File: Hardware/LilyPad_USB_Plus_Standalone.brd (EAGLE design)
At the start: 50.7 x 50.7 mm, 101 parts, among them J1 SEWTAP_LONG-2SIDE, J10 SEWTAP_LONG-2SIDE, J11 SEWTAP_LONG-2SIDE, J12 SEWTAP_LONG-2SIDE, J13 SEWTAP_LONG-2SIDE, J14 SEWTAP_LONG-2SIDE, J15 AMP FCI 10103594-0001LF, J2 SEWTAP_LONG-2SIDE, J3 SEWTAP_LONG-2SIDE, J4 SEWTAP_LONG-2SIDE, J5 SEWTAP_LONG-2SIDE, J6 SEWTAP_LONG-2SIDE, J7 SEWTAP_LONG-2SIDE, J8 SEWTAP_LONG-2SIDE, J9 SEWTAP_LONG-2SIDE, U1 MCP73831, U2 3.3V, U5 32U4, Y1 8MHz

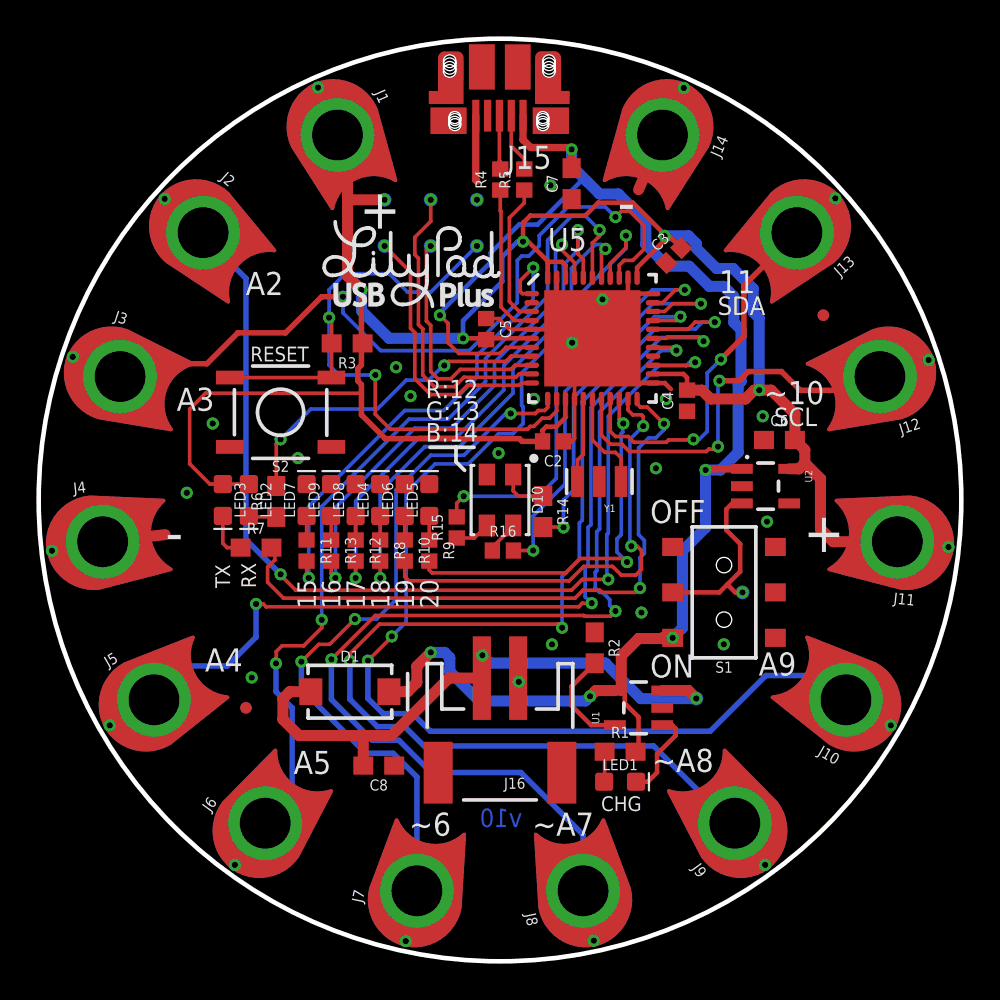
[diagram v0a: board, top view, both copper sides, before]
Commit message: Changes after double check
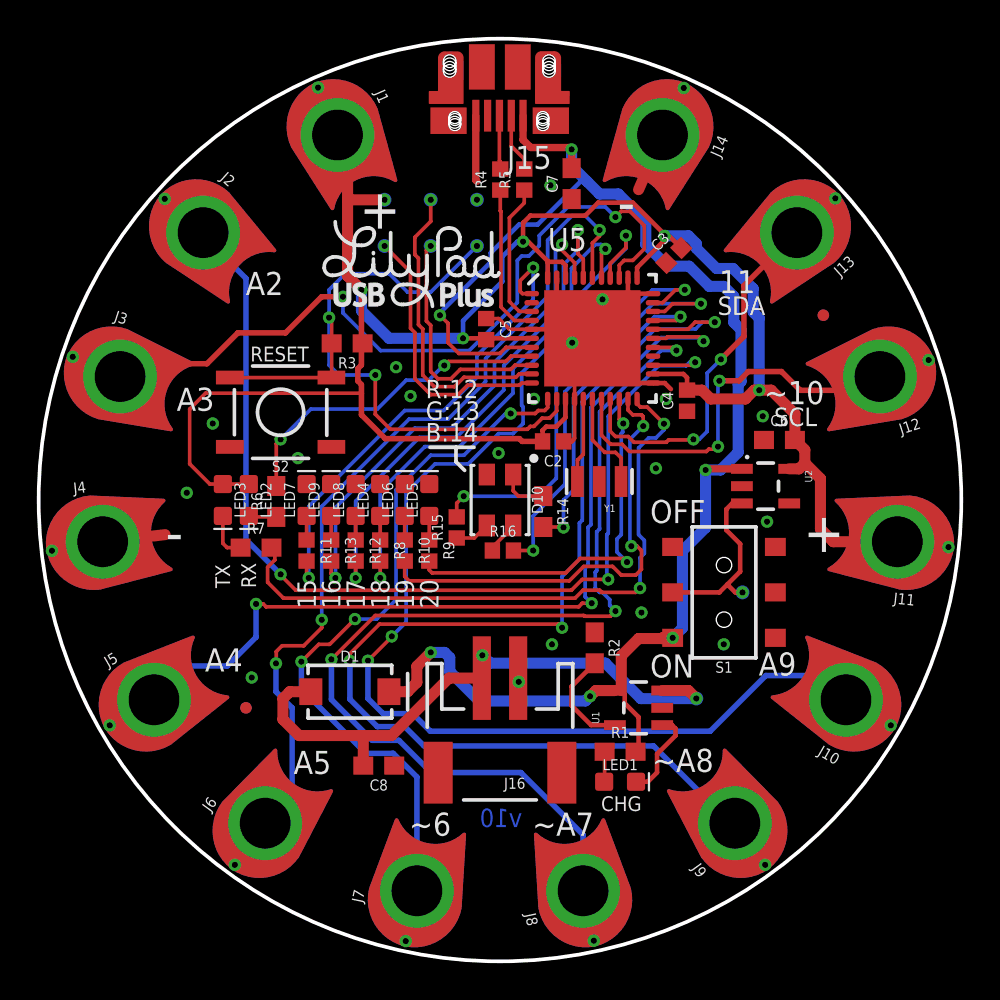
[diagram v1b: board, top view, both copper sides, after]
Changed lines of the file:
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@@
 <layer number="47" name="Measures" color="7" fill="1" visible="no" active="yes"/>
 <layer number="48" name="Document" color="7" fill="1" visible="no" active="no"/>
-<layer number="49" name="Reference" color="13" fill="1" visible="yes" active="yes"/>
+<layer number="49" name="Reference" color="13" fill="1" visible="no" active="yes"/>
 <layer number="50" name="dxf" color="7" fill="1" visible="no" active="no"/>
 <layer number="52" name="bDocu" color="7" fill="1" visible="no" active="no"/>
@@
 </polygon>
 <text x="-31.75" y="-13.97" size="1.778" layer="52" font="vector" rot="MR0">Revised by: Elias Santistevan</text>
-<circle x="25.4" y="25.4" radius="25.368509375" width="0.254" layer="20"/>
+<circle x="25.4" y="25.4" radius="25.368509375" width="0.2032" layer="20"/>
 <dimension x1="50.79999375" y1="25.4" x2="0.00000625" y2="25.4" x3="25.4" y3="60.96" textsize="1.778" textratio="15" layer="47" unit="inch"/>
 <text x="29.845" y="61.722" size="1.778" layer="47" font="vector" ratio="15">Inches</text>
